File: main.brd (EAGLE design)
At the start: 25.1 x 24.8 mm, 33 parts, among them IC1 ATTINY13A-SSH, T1A 2N4401, T1B NPN, T2A 2N4401, T2B NPN

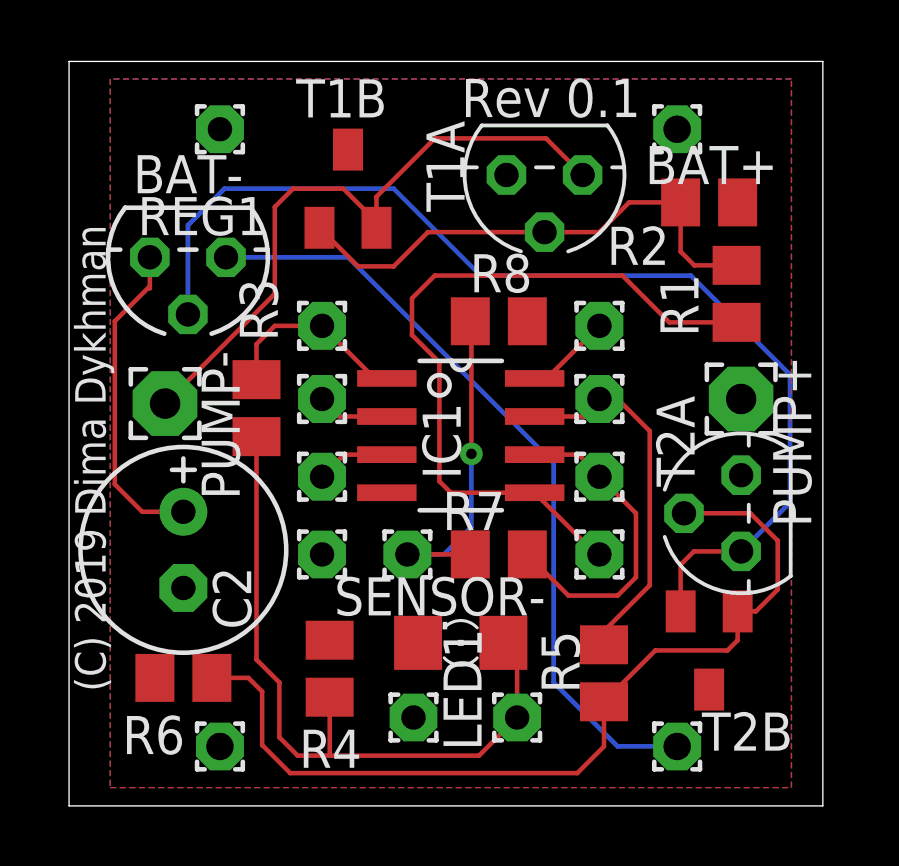
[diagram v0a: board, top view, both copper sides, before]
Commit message: a few more corrections
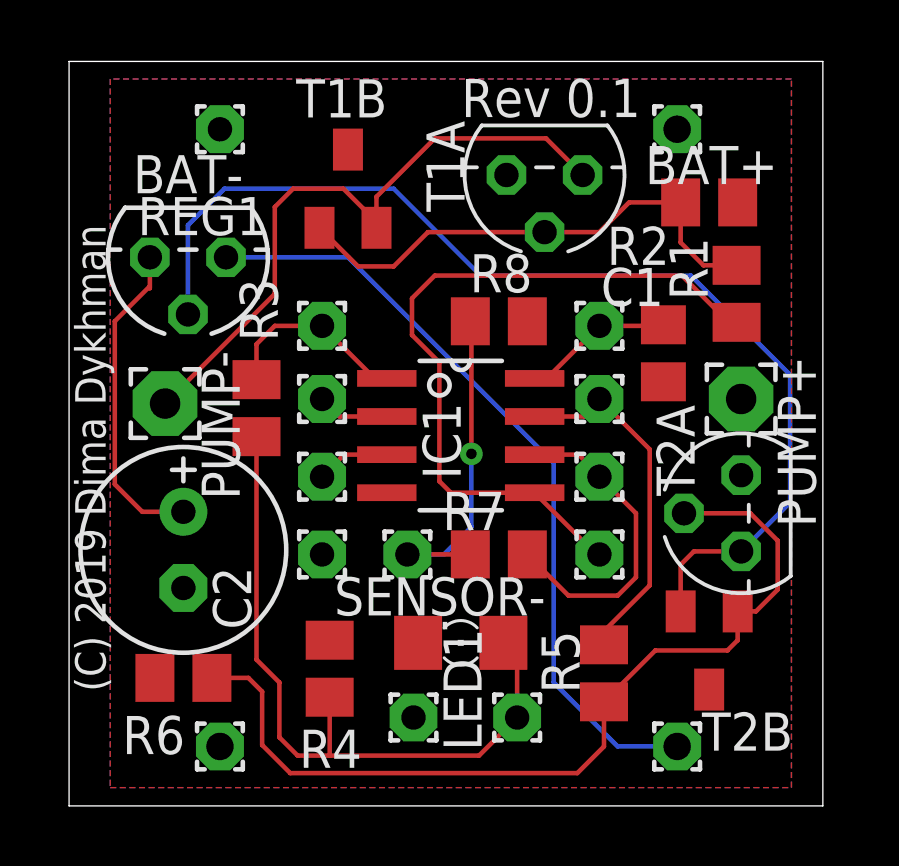
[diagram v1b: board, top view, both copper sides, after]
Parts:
- added C1: 100nF, rcl:C0805
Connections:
- net GND: now also C1.2
- net VCC: now also C1.1
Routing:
- net VCC: track 2.88 -> 5.03 mm
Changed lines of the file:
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@@
 </element>
 <element name="PUMP+" library="wirepad" library_urn="urn:adsk.eagle:library:412" package="2,15/1,0" package3d_urn="urn:adsk.eagle:package:30831/1" value="" x="22.86" y="14.0208" smashed="yes" rot="R90">
-<attribute name="NAME" x="25.1968" y="9.7536" size="1.27" layer="25" ratio="10" rot="R90"/>
+<attribute name="NAME" x="25.3492" y="9.7536" size="1.27" layer="25" ratio="10" rot="R90"/>
 <attribute name="VALUE" x="22.26" y="14.0208" size="0.0254" layer="27" rot="R90"/>
 </element>
@@
 </element>
 <element name="R1" library="resistor" library_urn="urn:adsk.eagle:library:348" package="M0805" package3d_urn="urn:adsk.eagle:package:23556/1" value="510" x="22.7076" y="17.526" smashed="yes" rot="R270">
-<attribute name="NAME" x="20.1676" y="18.1864" size="1.27" layer="25" rot="R270"/>
+<attribute name="NAME" x="20.4724" y="19.4056" size="1.27" layer="25" rot="R270"/>
 <attribute name="VALUE" x="20.1676" y="18.796" size="1.27" layer="27" rot="R270"/>
 </element>
@@
 </element>
 <element name="T2A" library="transistor" library_urn="urn:adsk.eagle:library:402" package="TO92" package3d_urn="urn:adsk.eagle:package:29893/2" value="2N4401" x="22.86" y="10.2108" smashed="yes" rot="R90">
-<attribute name="NAME" x="21.3106" y="11.0998" size="1.27" layer="25" ratio="10" rot="R90"/>
+<attribute name="NAME" x="21.3106" y="10.795" size="1.27" layer="25" ratio="10" rot="R90"/>
 <attribute name="VALUE" x="24.13" y="13.3858" size="1.27" layer="27" ratio="10" rot="R90"/>
 </element>
@@
 <attribute name="NAME" x="9.2964" y="6.8072" size="1.27" layer="25" ratio="10"/>
 <attribute name="VALUE" x="11.7348" y="9.4392" size="0.0254" layer="27"/>
+</element>
+<element name="C1" library="rcl" library_urn="urn:adsk.eagle:library:334" package="C0805" package3d_urn="urn:adsk.eagle:package:23617/2" value="100nF" x="20.2692" y="15.5448" smashed="yes" rot="R270">
+<attribute name="NAME" x="18.1864" y="17.1196" size="1.27" layer="25"/>
+<attribute name="SPICEPREFIX" value="C" x="20.2692" y="15.5448" size="1.778" layer="27" rot="R270" display="off"/>
+<attribute name="VALUE" x="17.7292" y="16.8148" size="1.27" layer="27" rot="R270"/>
 </element>
 </elements>
@@
 <contactref element="PAD2" pad="1"/>
 <contactref element="R8" pad="1"/>
+<contactref element="C1" pad="2"/>
 </signal>
 <signal name="N$1">
@@
 <wire x1="19.1262" y1="20.574" x2="18.1356" y2="19.5834" width="0.1524" layer="1"/>
 <wire x1="18.1356" y1="19.5834" x2="16.3068" y2="19.5834" width="0.1524" layer="1"/>
-<wire x1="22.7076" y1="18.476" x2="21.3004" y2="18.476" width="0.1524" layer="1"/>
-<wire x1="20.8432" y1="18.9332" x2="20.8432" y2="20.574" width="0.1524" layer="1"/>
-<wire x1="21.3004" y1="18.476" x2="20.8432" y2="18.9332" width="0.1524" layer="1"/>
+<wire x1="22.7076" y1="18.476" x2="21.6052" y2="18.476" width="0.1524" layer="1"/>
+<wire x1="20.8432" y1="19.238" x2="20.8432" y2="20.574" width="0.1524" layer="1"/>
+<wire x1="21.6052" y1="18.476" x2="20.8432" y2="19.238" width="0.1524" layer="1"/>
 </signal>
 <signal name="N$2">
@@
 <wire x1="19.812" y1="7.808" x2="18.288" y2="6.284" width="0.1524" layer="1"/>
 <wire x1="18.288" y1="5.8268" x2="18.288" y2="6.284" width="0.1524" layer="1"/>
-<wire x1="19.812" y1="12.954" x2="18.774228125" y2="13.991771875" width="0.1524" layer="1"/>
-<wire x1="18.774228125" y1="13.991771875" x2="18.1356" y2="14.0208" width="0.1524" layer="1"/>
-<wire x1="19.812" y1="7.808" x2="19.812" y2="12.954" width="0.1524" layer="1"/>
+<wire x1="19.812" y1="12.3444" x2="18.1356" y2="14.0208" width="0.1524" layer="1"/>
+<wire x1="19.812" y1="7.808" x2="19.812" y2="12.3444" width="0.1524" layer="1"/>
 </signal>
 <signal name="VCC">
@@
 <wire x1="15.9766" y1="14.7066" x2="16.383" y2="14.7066" width="0.1524" layer="1"/>
 <wire x1="16.383" y1="14.7066" x2="18.1356" y2="16.4592" width="0.1524" layer="1"/>
+<contactref element="C1" pad="1"/>
+<wire x1="20.2692" y1="16.4948" x2="20.2336" y2="16.4592" width="0.1524" layer="1"/>
+<wire x1="20.2336" y1="16.4592" x2="18.1356" y2="16.4592" width="0.1524" layer="1"/>
 </signal>
 <signal name="SENSOR">
@@
 <wire x1="15.9766" y1="10.8966" x2="13.1826" y2="10.8966" width="0.1524" layer="1"/>
 <wire x1="13.1826" y1="10.8966" x2="12.8016" y2="11.2776" width="0.1524" layer="1"/>
-<wire x1="12.6492" y1="18.1356" x2="18.90370625" y2="18.1356" width="0.1524" layer="1"/>
+<wire x1="12.6492" y1="18.1356" x2="20.88490625" y2="18.1356" width="0.1524" layer="1"/>
 <wire x1="11.8872" y1="17.3736" x2="12.6492" y2="18.1356" width="0.1524" layer="1"/>
-<wire x1="18.90370625" y1="18.1356" x2="20.46330625" y2="16.576" width="0.1524" layer="1"/>
-<wire x1="20.46330625" y1="16.576" x2="22.7076" y2="16.576" width="0.1524" layer="1"/>
+<wire x1="22.7076" y1="16.576" x2="22.44450625" y2="16.576" width="0.1524" layer="1"/>
+<wire x1="22.44450625" y1="16.576" x2="20.88490625" y2="18.1356" width="0.1524" layer="1"/>
 <wire x1="12.8016" y1="11.2776" x2="12.8016" y2="15.24" width="0.1524" layer="1"/>
 <wire x1="12.8016" y1="15.24" x2="11.8872" y2="16.1544" width="0.1524" layer="1"/>
